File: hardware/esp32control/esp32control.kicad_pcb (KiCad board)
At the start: 2 copper layers, 67.6 x 85.9 mm, 86 parts, among them J1 Conn_02x10_Odd_Even, Q1 BSS138, Q2 BSS138, Q3 BSS138, Q4 BSS138, Q5 BSS138, Q6 BSS138, Q7 MMBT3904, Q8 MMBT3904, SW1 Boot, SW2 Reset, U1 ESP32-WROOM, U10 LTV-354T, U11 HUT4, U12 LM1117-3.3, U13 RV-8523-C3, U2 AQY212, U3 AQY212, U4 LM2675M-5, U5 LTV-354T, U6 AQY212, U7 AQY212, U8 LTV-354T, U9 LTV-354T

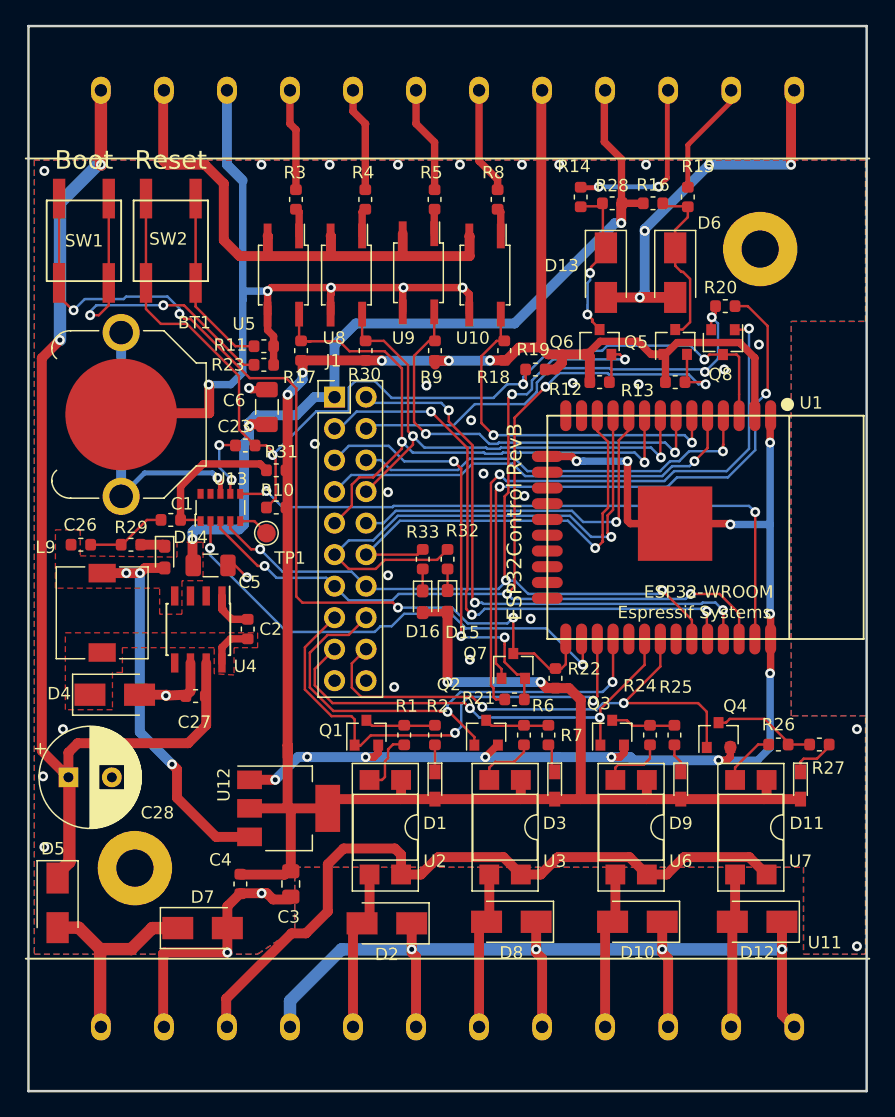
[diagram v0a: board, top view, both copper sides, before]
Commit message: kicad6 update
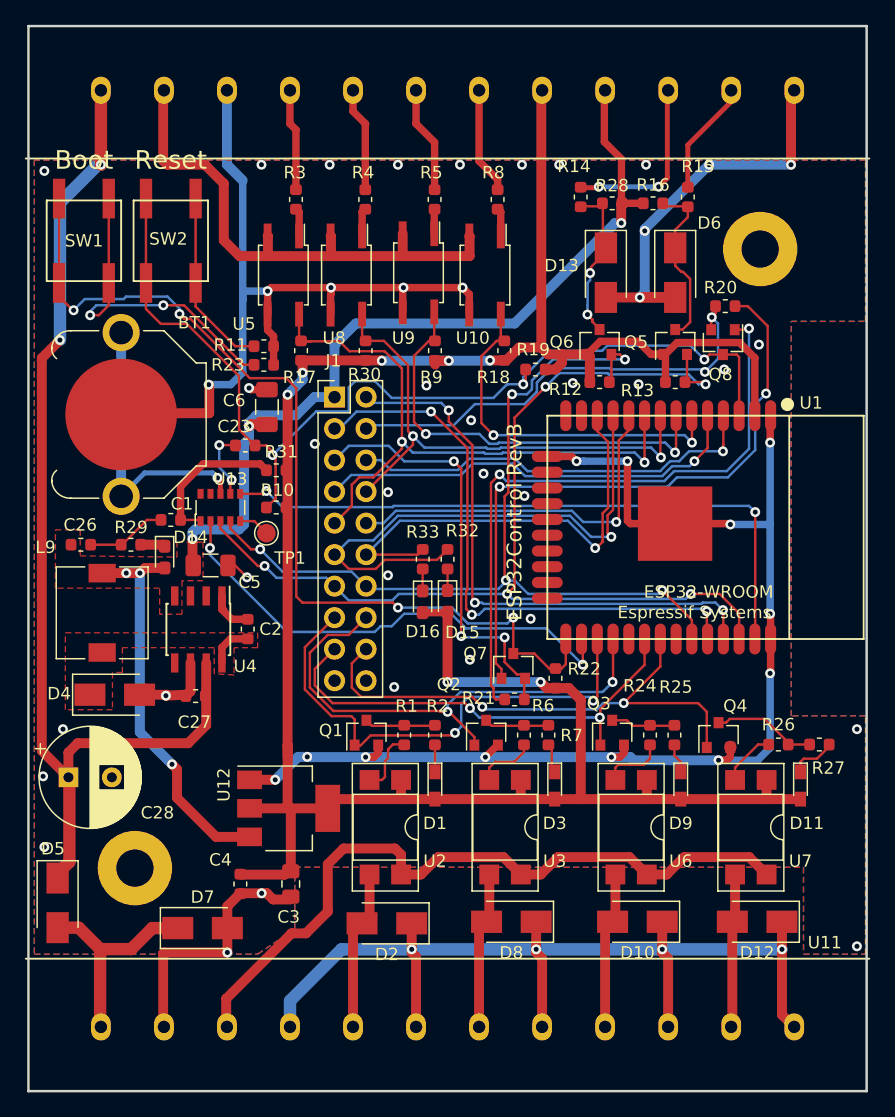
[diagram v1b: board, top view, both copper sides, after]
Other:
- net class Default removed
